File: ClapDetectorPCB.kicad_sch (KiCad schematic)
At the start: 0 parts

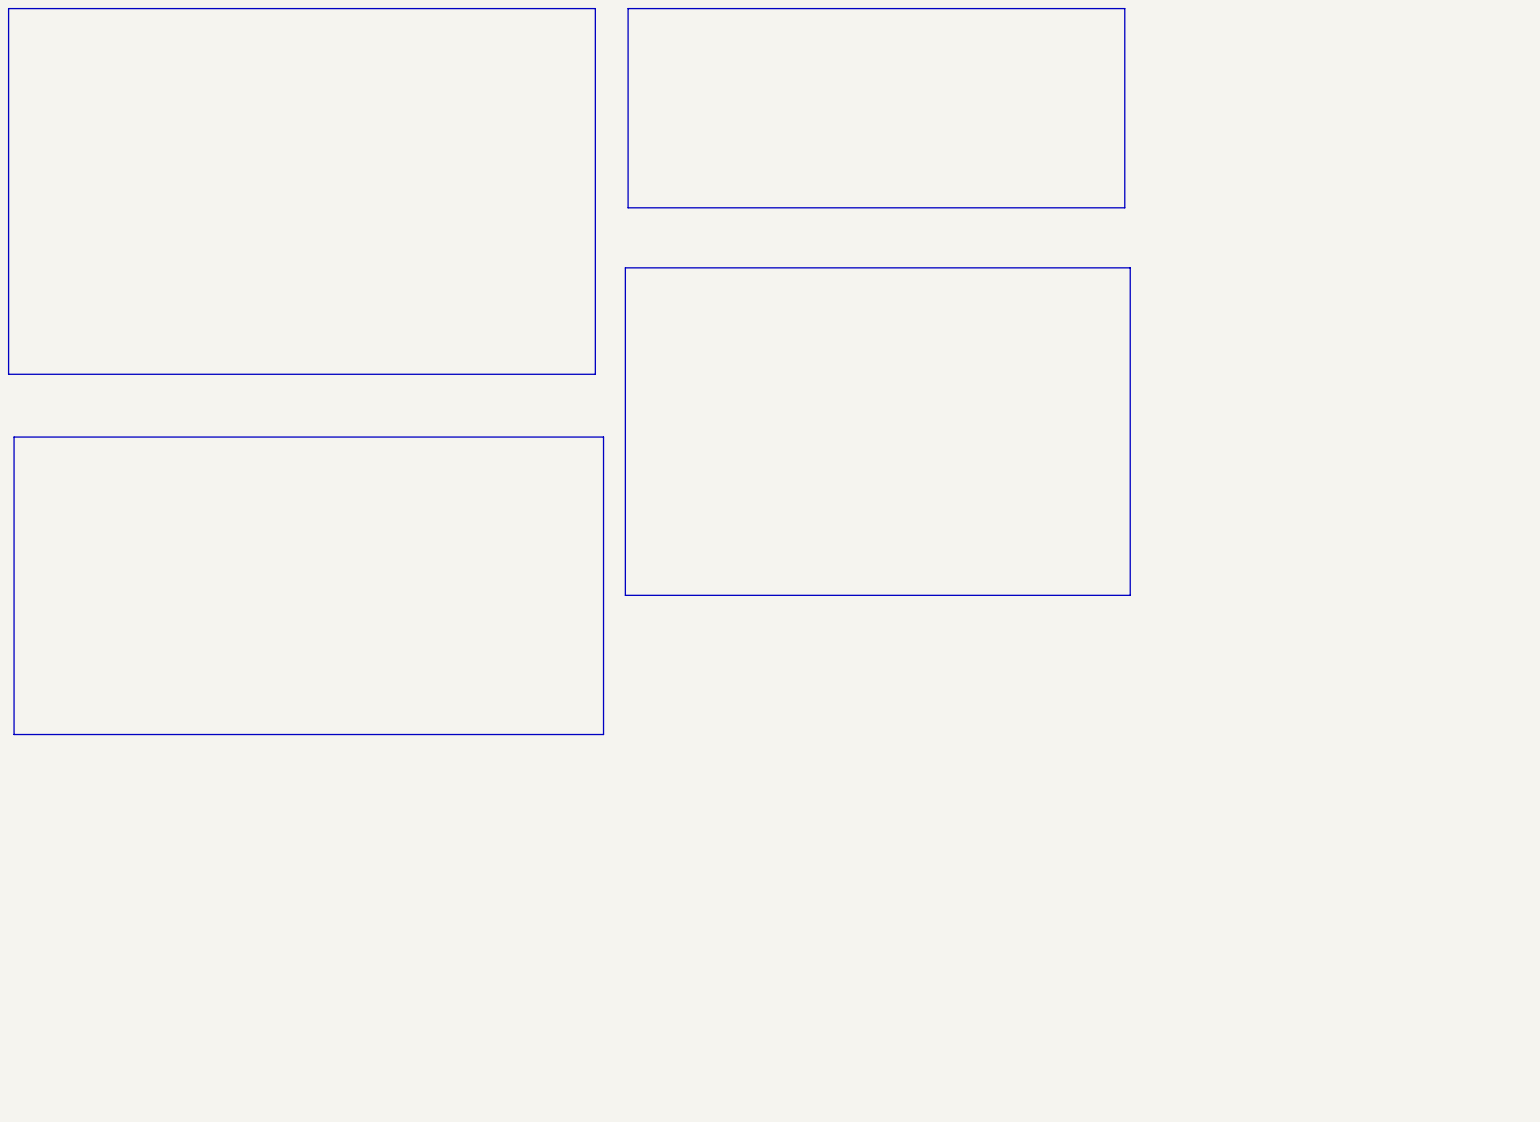
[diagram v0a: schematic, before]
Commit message: hi2
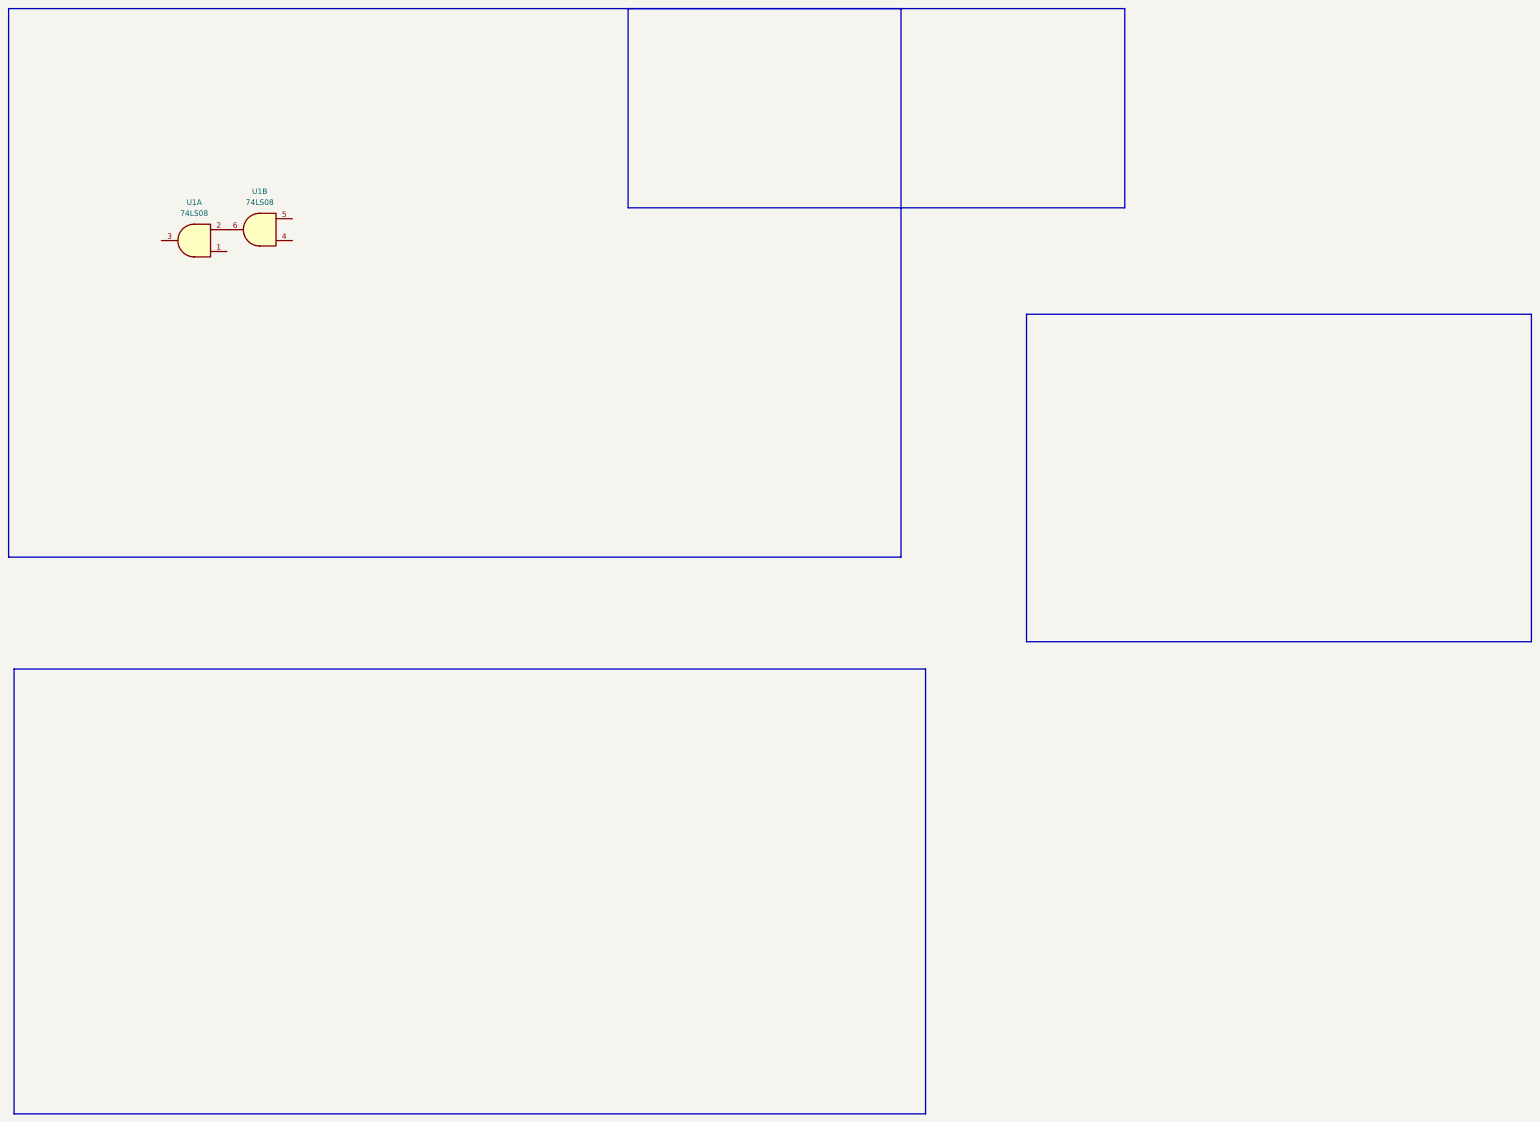
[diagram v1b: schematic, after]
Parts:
- added U1: 74LS08, symbol 74xx:74LS08
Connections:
- new net: U1.2, U1.6
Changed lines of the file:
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@@
 	(generator "eeschema")
 	(generator_version "10.0")
-	(paper "A4")
+	(paper "A3")
 	(rectangle
 		(start 17.78 22.225)
-		(end 154.305 107.315)
-		(stroke
-			(width 0)
-			(type default)
-		)
-		(fill
-			(type none)
-		)
-	)
-	(rectangle
-		(start 19.05 121.92)
-		(end 156.21 191.135)
+		(end 225.425 149.86)
+		(stroke
+			(width 0)
+			(type default)
+		)
+		(fill
+			(type none)
+		)
+	)
+	(rectangle
+		(start 19.05 175.895)
+		(end 231.14 279.4)
 		(stroke
 			(width 0)
@@
 	)
 	(rectangle
-		(start 161.29 82.55)
-		(end 278.765 158.75)
-		(stroke
-			(width 0)
-			(type default)
-		)
-		(fill
-			(type none)
-		)
-	)
+		(start 254.635 93.345)
+		(end 372.11 169.545)
+		(stroke
+			(width 0)
+			(type default)
+		)
+		(fill
+			(type none)
+		)
+	)
+	(symbol
+		(lib_id "74xx:74LS08")
+		(at 76.2 73.66 180)
+		(unit 2)
+		(body_style 1)
+		(exclude_from_sim no)
+		(in_bom yes)
+		(on_board yes)
+		(in_pos_files yes)
+		(dnp no)
+		(fields_autoplaced yes)
+		(property "Reference" "U1"
+			(at 76.2083 64.77 0)
+			(show_name no)
+			(do_not_autoplace no)
+			(effects
+				(font
+					(size 1.27 1.27)
+				)
+			)
+		)
+		(property "Value" "74LS08"
+			(at 76.2083 67.31 0)
+			(show_name no)
+			(do_not_autoplace no)
+			(effects
+				(font
+					(size 1.27 1.27)
+				)
+			)
+		)
+		(property "Footprint" ""
+			(at 76.2 73.66 0)
+			(hide yes)
+			(show_name no)
+			(do_not_autoplace no)
+			(effects
+				(font
+					(size 1.27 1.27)
+				)
+			)
+		)
+		(property "Datasheet" "http://www.ti.com/lit/gpn/sn74LS08"
+			(at 76.2 73.66 0)
+			(hide yes)
+			(show_name no)
+			(do_not_autoplace no)
+			(effects
+				(font
+					(size 1.27 1.27)
+				)
+			)
+		)
+		(property "Description" "Quad And2"
+			(at 76.2 73.66 0)
+			(hide yes)
+			(show_name no)
+			(do_not_autoplace no)
+			(effects
+				(font
+					(size 1.27 1.27)
+				)
+			)
+		)
+		(pin "8"
+		)
+		(pin "9"
+		)
+		(pin "10"
+		)
+		(pin "1"
+		)
+		(pin "3"
+		)
+		(pin "4"
+		)
+		(pin "5"
+		)
+		(pin "6"
+		)
+		(pin "2"
+		)
+		(pin "14"
+		)
+		(pin "7"
+		)
+		(pin "12"
+		)
+		(pin "13"
+		)
+		(pin "11"
+		)
+		(instances
+			(project "ClapDetectorPCB"
+				(path "/a9e28604-8006-42a0-85f5-c1dddeb9dfef"
+					(reference "U1")
+					(unit 2)
+				)
+			)
+		)
+	)
+	(symbol
+		(lib_id "74xx:74LS08")
+		(at 60.96 76.2 180)
+		(unit 1)
+		(body_style 1)
+		(exclude_from_sim no)
+		(in_bom yes)
+		(on_board yes)
+		(in_pos_files yes)
+		(dnp no)
+		(fields_autoplaced yes)
+		(property "Reference" "U1"
+			(at 60.9683 67.31 0)
+			(show_name no)
+			(do_not_autoplace no)
+			(effects
+				(font
+					(size 1.27 1.27)
+				)
+			)
+		)
+		(property "Value" "74LS08"
+			(at 60.9683 69.85 0)
+			(show_name no)
+			(do_not_autoplace no)
+			(effects
+				(font
+					(size 1.27 1.27)
+				)
+			)
+		)
+		(property "Footprint" ""
+			(at 60.96 76.2 0)
+			(hide yes)
+			(show_name no)
+			(do_not_autoplace no)
+			(effects
+				(font
+					(size 1.27 1.27)
+				)
+			)
+		)
+		(property "Datasheet" "http://www.ti.com/lit/gpn/sn74LS08"
+			(at 60.96 76.2 0)
+			(hide yes)
+			(show_name no)
+			(do_not_autoplace no)
+			(effects
+				(font
+					(size 1.27 1.27)
+				)
+			)
+		)
+		(property "Description" "Quad And2"
+			(at 60.96 76.2 0)
+			(hide yes)
+			(show_name no)
+			(do_not_autoplace no)
+			(effects
+				(font
+					(size 1.27 1.27)
+				)
+			)
+		)
+		(pin "8"
+		)
+		(pin "9"
+		)
+		(pin "10"
+		)
+		(pin "1"
+		)
+		(pin "3"
+		)
+		(pin "4"
+		)
+		(pin "5"
+		)
+		(pin "6"
+		)
+		(pin "2"
+		)
+		(pin "14"
+		)
+		(pin "7"
+		)
+		(pin "12"
+		)
+		(pin "13"
+		)
+		(pin "11"
+		)
+		(instances
+			(project "ClapDetectorPCB"
+				(path "/a9e28604-8006-42a0-85f5-c1dddeb9dfef"
+					(reference "U1")
+					(unit 1)
+				)
+			)
+		)
+	)
